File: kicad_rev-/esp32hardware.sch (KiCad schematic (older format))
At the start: 40 parts, among them U1 TS4231, U2 TS4231, U3 TS4231, U4 TS4231, U5 TS4231, U6 TS4231, U7 TS4231, U8 TS4231

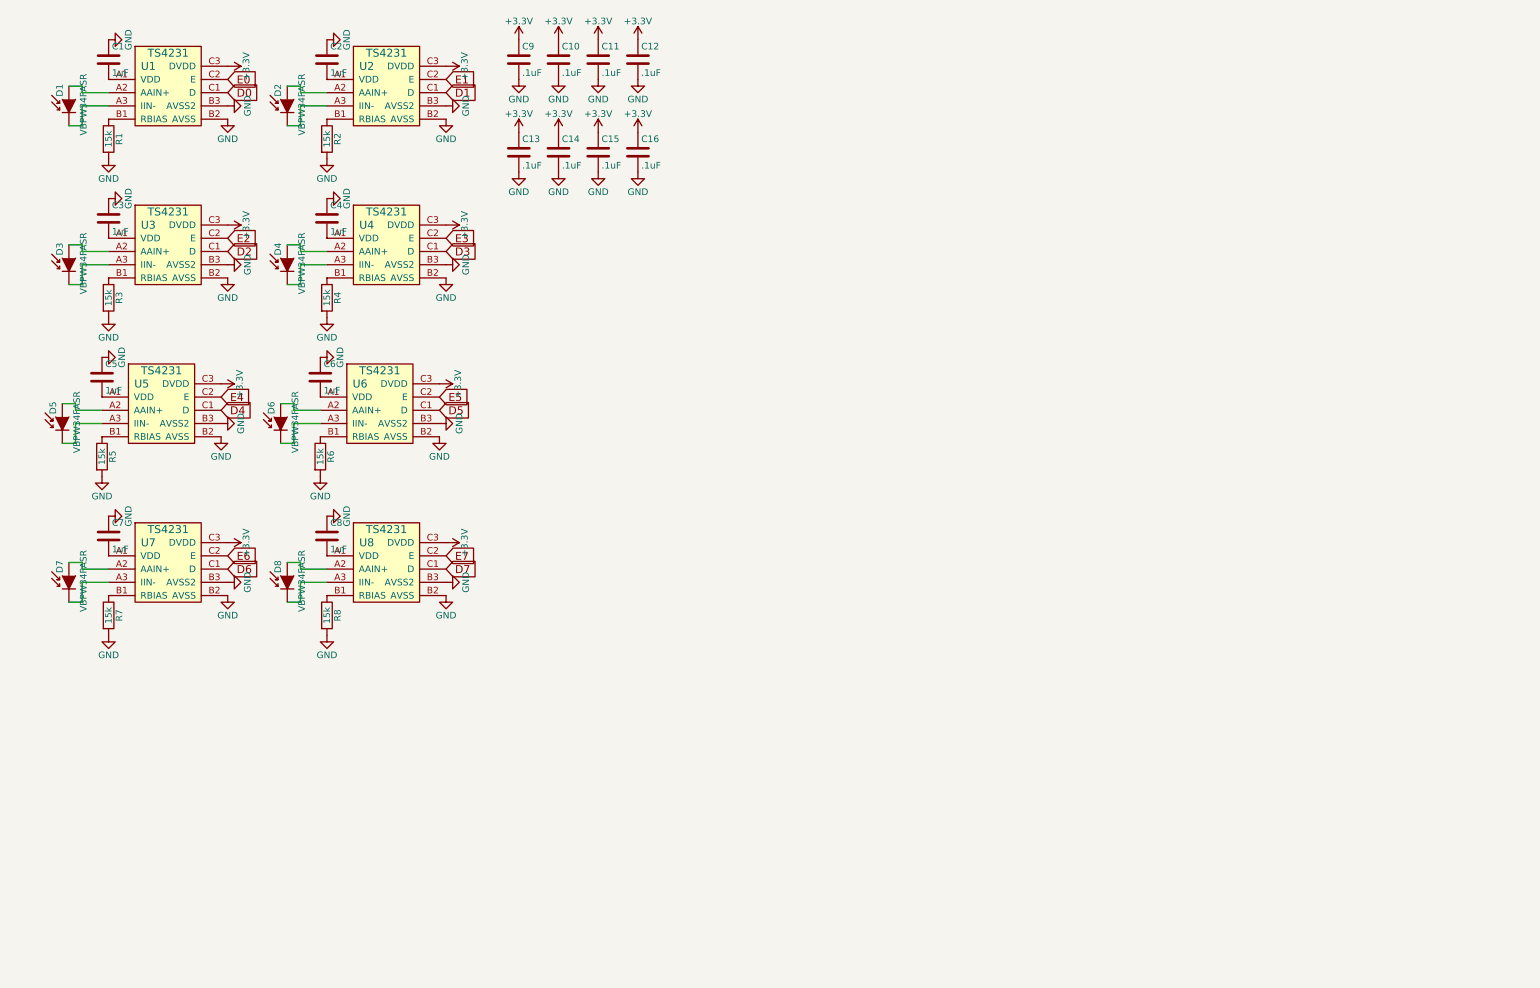
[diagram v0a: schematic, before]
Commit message: More progress...
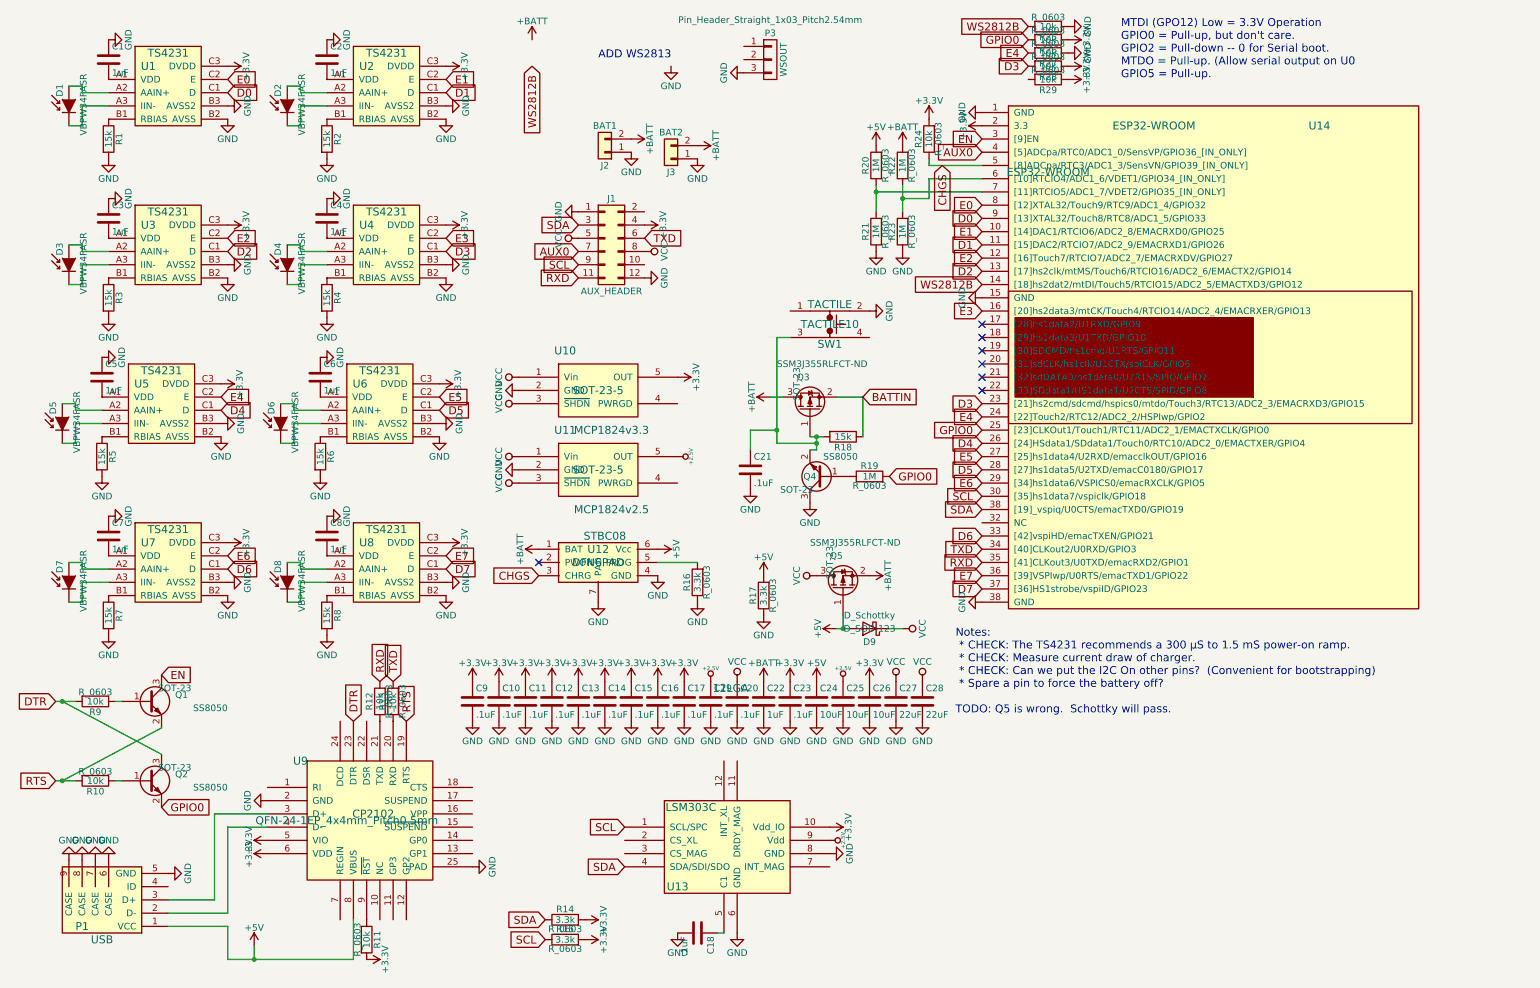
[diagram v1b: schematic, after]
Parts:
- added C17, C18, C19, C20, C21, C23: .1uF, C_0603, symbol C
- added C22: 1uF, C_0603, symbol C
- added C24, C25, C26: 10uF, C_0603, symbol C
- added C27, C28: 22uF, C_0603, symbol C
- added D9: D_Schottky, D_SOD-123, symbol D_Schottky
- added J1: AUX_HEADER, RIBBON12SMT, symbol Conn_02x06_Odd_Even
- added J2: BAT1, Pin_Header_Straight_1x02_Pitch2.54mm, symbol Conn_01x02
- added J3: BAT2, Pin_Header_Straight_1x02_Pitch2.54mm, symbol Conn_01x02
- added P1: USB, USBMicroB-10118194-0001LF, symbol USBMicroB-10118194-0001LF
- added P3: WSOUT, Pin_Header_Straight_1x03_Pitch2.54mm, symbol CONN_01X03
- added Q1, Q2, Q4: SS8050, SOT-23, symbol Q_NPN_BEC
- added Q3, Q5: SSM3J355RLFCT-ND, SOT-23, symbol Q_PMOS_GSD
- added R10, R11, R12, R13, R24, R25, R26, R27, R28, R29, R9: 10k, R_0603, symbol R
- added R14, R15, R16, R17: 3.3k, R_0603, symbol R
- added R18: 15k, R_0603, symbol R
- added R19, R20, R21, R22, R23: 1M, R_0603, symbol R
- added SW1: TACTILE, TACTILE10, symbol TACTILE
- added U10: MCP1824v3.3, SOT-23-5, symbol MCP1824
- added U11: MCP1824v2.5, SOT-23-5, symbol MCP1824
- added U12: STBC08, DFN6PAD, symbol STBC08-BATTCHARGER
- added U13: LSM303C, 12LGA, symbol LSM303C
- added U14: ESP32-WROOM, ESP32-WROOM, symbol ESP32-WROOM
- added U9: CP2102, QFN-24-1EP_4x4mm_Pitch0.5mm, symbol CP2104
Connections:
- net +3V3: now also C17.1, C23.1, C26.1, J1.4 (Pin_4), R11.2, R14.2, R15.2, R24.2, R26.1, R28.1, R29.1, U10.5 (OUT), U13.10 (Vdd_IO), U14.2 (3.3), U9.5 (VIO), U9.6 (VDD)
- net D0: now also U14.9 ([13]XTAL32/Touch8/RTC8/ADC1_5/GPIO33)
- net D1: now also U14.11 ([15]DAC2/RTCIO7/ADC2_9/EMACRXD1/GPIO26)
- net D2: now also U14.13 ([17]hs2clk/mtMS/Touch6/RTCIO16/ADC2_6/EMACTX2/GPIO14)
- net D3: now also R28.2, U14.23 ([21]hs2cmd/sdcmd/hspics0/mtdo/Touch3/RTC13/ADC2_3/EMACRXD3/GPIO15)
- net D4: now also U14.26 ([24]HSdata1/SDdata1/Touch0/RTC10/ADC2_0/EMACTXER/GPIO4)
- net D5: now also U14.28 ([27]hs1data5/U2TXD/emacC0180/GPIO17)
- net D6: now also U14.33 ([42]vspiHD/emacTXEN/GPIO21)
- net D7: now also U14.37 ([36]HS1strobe/vspiID/GPIO23)
- net E0: now also U14.8 ([12]XTAL32/Touch9/RTC9/ADC1_4/GPIO32)
- net E1: now also U14.10 ([14]DAC1/RTCIO6/ADC2_8/EMACRXD0/GPIO25)
- net E2: now also U14.12 ([16]Touch7/RTCIO7/ADC2_7/EMACRXDV/GPIO27)
- net E3: now also U14.16 ([20]hs2data3/mtCK/Touch4/RTCIO14/ADC2_4/EMACRXER/GPIO13)
- net E4: now also R27.2, U14.24 ([22]Touch2/RTC12/ADC2_2/HSPIwp/GPIO2)
- net E5: now also U14.27 ([25]hs1data4/U2RXD/emacclkOUT/GPIO16)
- net E6: now also U14.29 ([34]hs1data6/VSPICS0/emacRXCLK/GPIO5)
- net E7: now also U14.36 ([39]VSPIwp/U0RTS/emacTXD1/GPIO22)
- net GND: now also C17.2, C18.2, C19.2, C20.2, C21.2, C22.2, C23.2, C24.2, C25.2, C26.2, C27.2, C28.2, J1.1 (Pin_1), J1.12 (Pin_12), J2.1 (Pin_1), J3.1 (Pin_1), P1.5 (GND), P1.6 (CASE), P1.7 (CASE), P1.8 (CASE), P1.9 (CASE), P3.3 (P3), Q4.3 (C), R16.1, R17.1, R21.1, R23.1, R25.1, R27.1, SW1.2, U10.2 (GND), U11.2 (GND), U12.4 (GND), U12.7 (PAD), U13.6 (GND), U13.8 (GND), U14.1 (GND), U14.15 (GND), U14.38 (GND), U9.2 (GND), U9.25 (PAD)
- new net: R11.1, U9.9 (~RST~)
- new net: P1.2 (D-), U9.4 (D-)
- new net: P1.3 (D+), U9.3 (D+)
- new net: R13.1, U9.20 (RXD)
- new net: R12.1, U9.21 (TXD)
- new net: Q1.1 (B), R9.1
- new net: Q2.1 (B), R10.1
- new net: R22.1, R23.2, U14.6 ([10]RTCIO4/ADC1_6/VDET1/GPIO34_[IN_ONLY])
- new net: R20.1, R21.2, U14.7 ([11]RTCIO5/ADC1_7/VDET2/GPIO35_[IN_ONLY])
- new net: C18.1, U13.5 (C1)
- new net: R16.2, U12.5 (PROG)
- new net: C21.1, Q3.1 (G), Q4.2 (E), R18.2, SW1.3
- new net: Q4.1 (B), R19.1
- new net +2.5V: C19.1, C25.1, U11.5 (OUT), U13.9 (Vdd)
- new net +5V: C24.1, D9.2 (A), P1.1 (VCC), Q5.1 (G), R17.2, R20.2, U12.6 (Vcc), U9.8 (VBUS)
- new net +BATT: C22.1, J2.2 (Pin_2), J3.2 (Pin_2), Q3.3 (D), Q5.2 (S), R22.2, U12.1 (BAT)
- new net AUX0: J1.7 (Pin_7), U14.4 ([5]ADCpa/RTC0/ADC1_0/SensVP/GPIO36_[IN_ONLY])
- new net BATTIN: Q3.2 (S), R18.1
- new net CHGS: R24.1, U12.3 (CHRG), U14.5 ([8]ADCpa/RTC3/ADC1_3/SensVN/GPIO39_[IN_ONLY])
- new net DTR: Q2.3 (C), R9.2, U9.23 (DTR)
- new net EN: Q1.3 (C), U14.3 ([9]EN)
- new net GPIO0: Q2.2 (E), R19.2, R26.2, U14.25 ([23]CLKOut1/Touch1/RTC11/ADC2_1/EMACTXCLK/GPIO0)
- new net RTS: Q1.2 (E), R10.2, U9.19 (RTS)
- new net RXD: J1.11 (Pin_11), R12.2, U14.35 ([41]CLKout3/U0TXD/emacRXD2/GPIO1)
- new net SCL: J1.9 (Pin_9), R15.1, U13.1 (SCL/SPC), U14.30 ([35]hs1data7/vspiclk/GPIO18)
- new net SDA: J1.3 (Pin_3), R14.1, U13.4 (SDA/SDI/SDO), U14.38 (GND)
- new net TXD: J1.6 (Pin_6), R13.2, U14.34 ([40]CLKout2/U0RXD/GPIO3)
- new net VCC: C20.1, C27.1, C28.1, D9.1 (K), J1.5 (Pin_5), J1.8 (Pin_8), Q5.3 (D), U10.1 (Vin), U10.3 (~SHDN), U11.1 (Vin), U11.3 (~SHDN)
- new net WS2812B: R25.2, U14.14 ([18]hs2dat2/mtDI/Touch5/RTCIO15/ADC2_5/EMACTXD3/GPIO12)
- no-connect marks 0 -> 7
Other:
- note added: "ADD WS2813"
- note added: "MTDI (GPO12) Low = 3.3V Operation\nGPIO0 = Pull-up, but don't care.\nGPIO2 = Pull-down -- 0 for Serial boot.\nMTDO = Pull-up. (Allow serial output on U0\nGPIO5 = Pull-up."
- note added: "Notes:\n * CHECK: The TS4231 recommends a 300 μS to 1.5 mS power-on ramp.\n * CHECK: Measure current draw of charger.\n * CHECK: Can we put the I2C On other pins? (Convenient for bootstrapping)\n * Spare a pin to force the battery off?\n\nTODO: Q5 is wrong. Schottky will pass."
- moved on the sheet: C10, C11, C12, C13, C14, C15, C16, C9
